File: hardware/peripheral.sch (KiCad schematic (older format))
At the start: 51 parts, among them J11 Screw_Terminal_01x04, J60 USB_C_Receptacle, J62 Conn_01x02, J71 Conn_01x02, J72 Conn_01x02, J73 Conn_01x02, Q2 AO3400, Q4 AON7418, Q5 AON7418, U5 MAX6675, U6 IR4427S

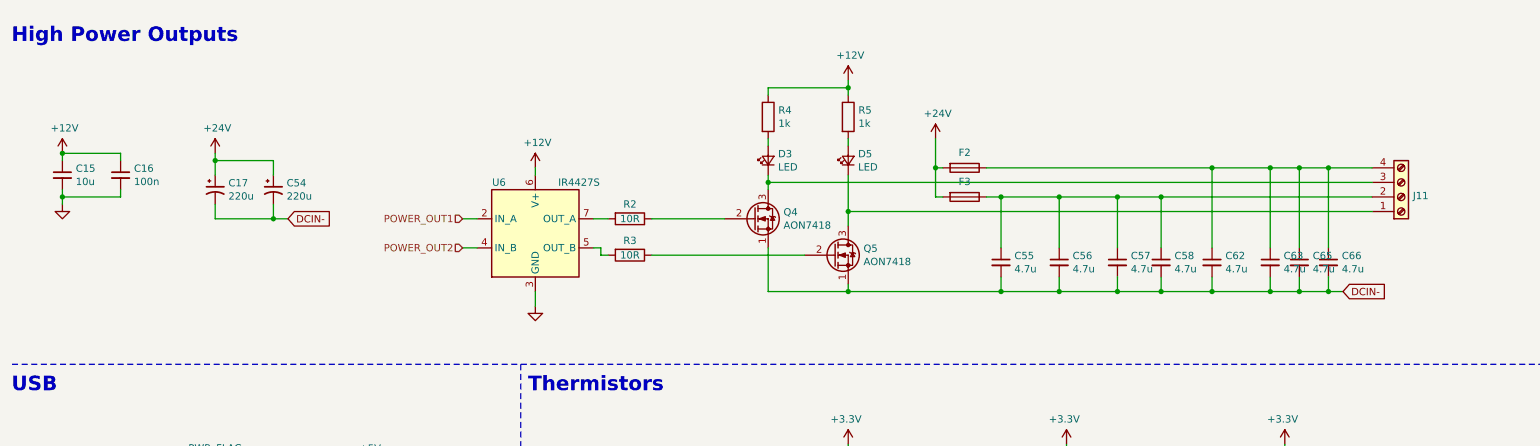
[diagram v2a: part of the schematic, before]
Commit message: routing
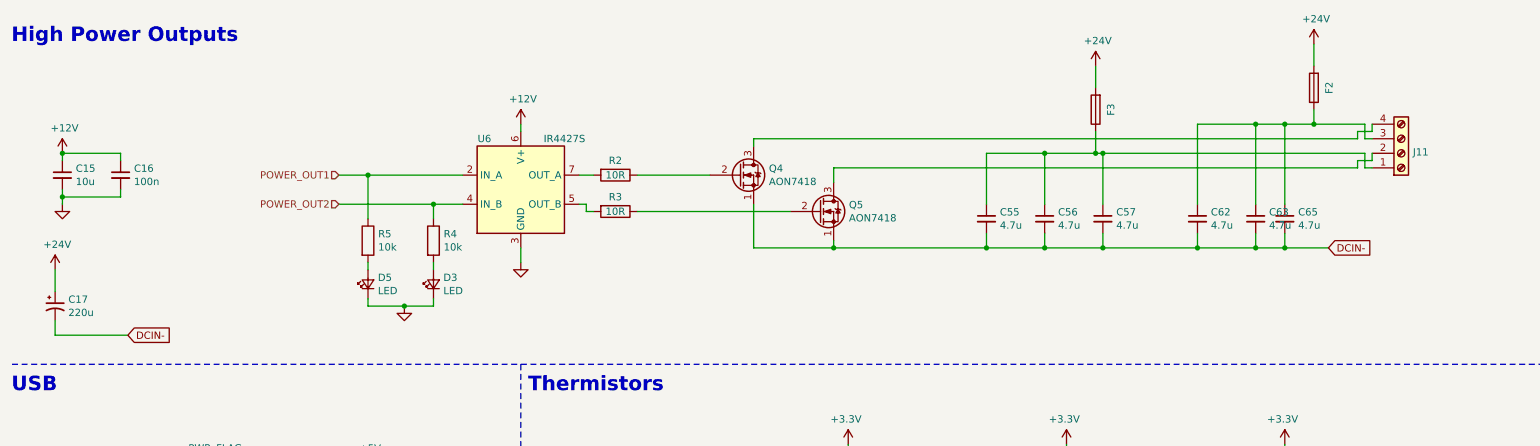
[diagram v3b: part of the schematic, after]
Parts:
- removed C54: 220u, Capacitor_SMD:CP_Elec_6.3x7.7, symbol Device:CP1_Small
- removed C58, C66: 4.7u, _Generic:1210_CAP, symbol Device:C_Small
- R4, R5: value 1k -> 10k
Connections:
- net +12V: no longer R4.1, R5.1
- net GND: now also D3.1 (K), D5.1 (K)
- net POWER_OUT1: now also R5.1
- net POWER_OUT2: now also R4.1
- net at C55.1, C56.1, C57.1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: now also J11.1 (Pin_1); no longer J11.2 (Pin_2)
- net at C62.1, C63.1, C65.1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: now also J11.3 (Pin_3); no longer J11.4 (Pin_4)
- new net: J11.2 (Pin_2), Q5.3 (D)
- new net: J11.4 (Pin_4), Q4.3 (D)
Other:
- moved on the sheet: C17, C55, C56, C57, C62, C63, C65, D3, D5, F2, F3, J11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
